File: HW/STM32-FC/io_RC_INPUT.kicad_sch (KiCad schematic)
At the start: 9 parts, among them J6 PWM_Conn_3x14, J7 ZH 1.5mm 4P, J8 ZH 1.5mm 3P, Q2 S9013

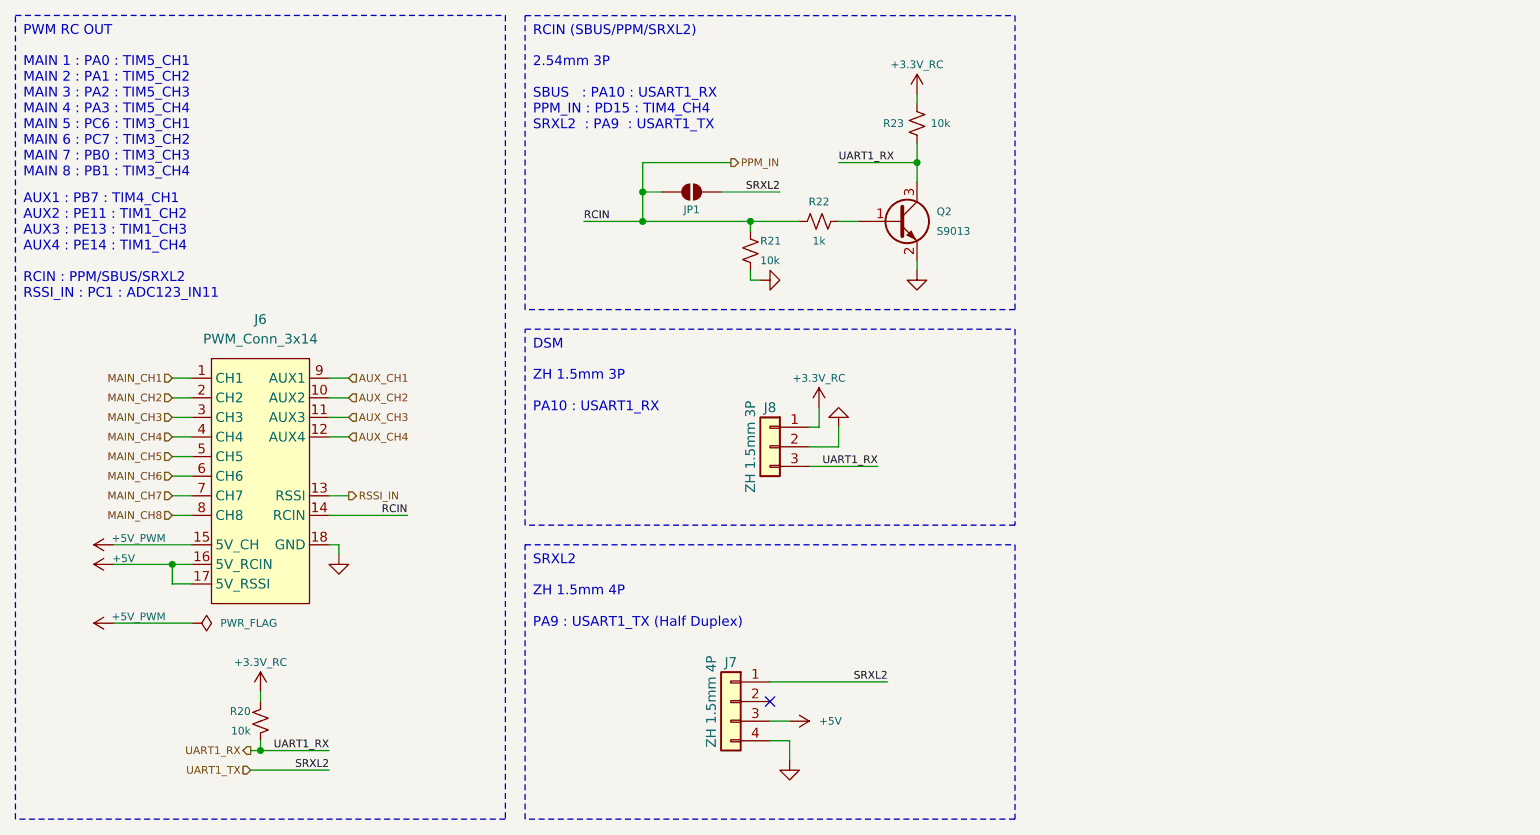
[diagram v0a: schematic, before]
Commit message: Log add. backup
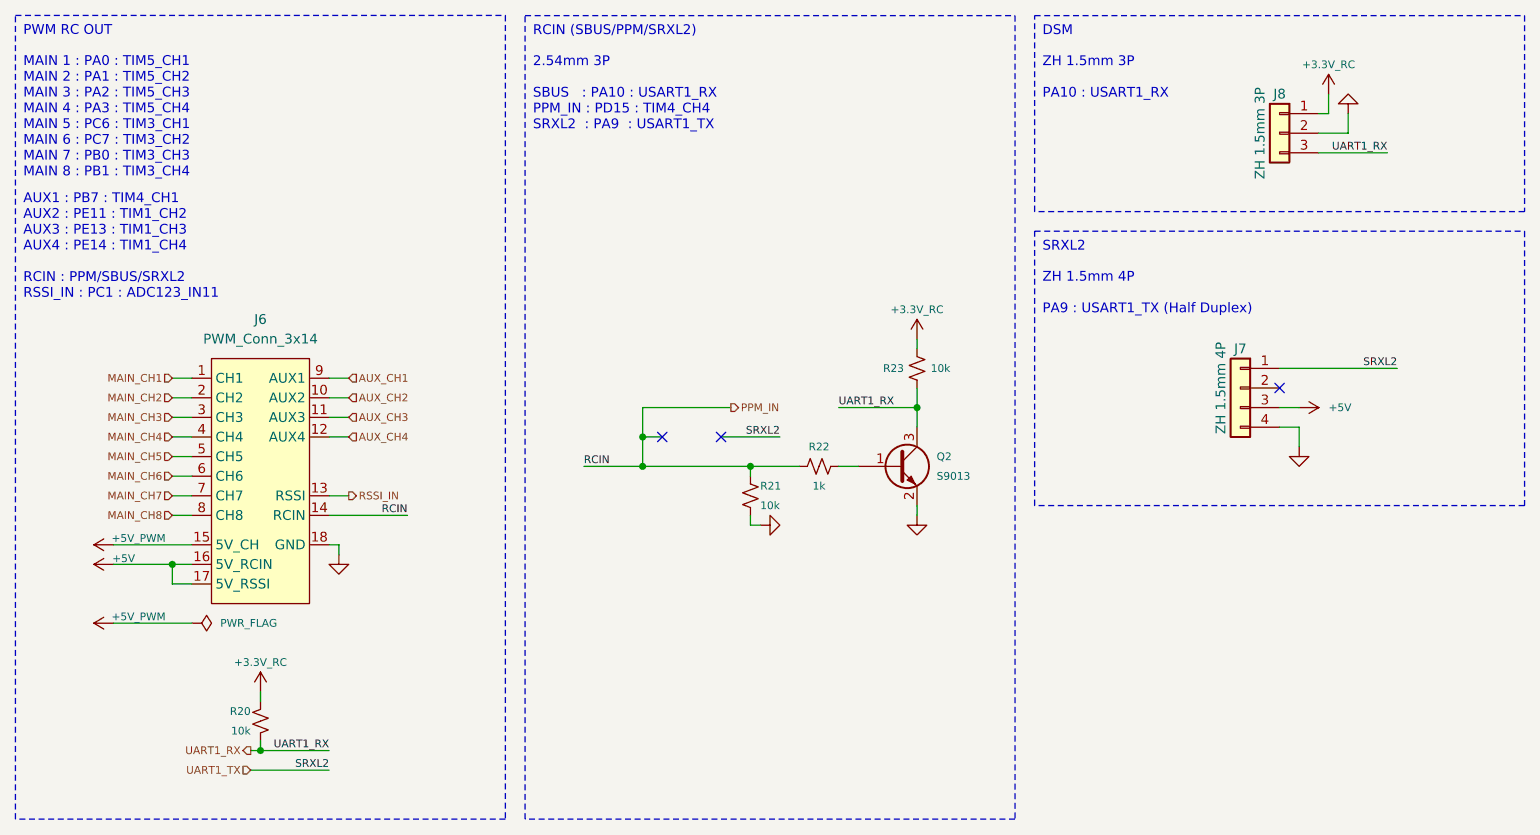
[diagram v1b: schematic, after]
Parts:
- removed JP1: SolderJumper_2_Open, Jumper:SolderJumper-2_P1.3mm_Open_TrianglePad1.0x1.5mm, symbol Jumper:SolderJumper_2_Open
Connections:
- no-connect marks 1 -> 3
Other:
- moved on the sheet: J7, J8, Q2, R21, R22, R23
